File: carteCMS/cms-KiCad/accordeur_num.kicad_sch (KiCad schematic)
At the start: 16 parts, among them J2 Conn_01x16, J3 AVR-ISP-6, SW2 MCIPTG23K-V, SW3 MCIPTG23K-V, SW4 MCIPTG23K-V, U5 HP, U6 ATmega8U2-A, Y2 Crystal

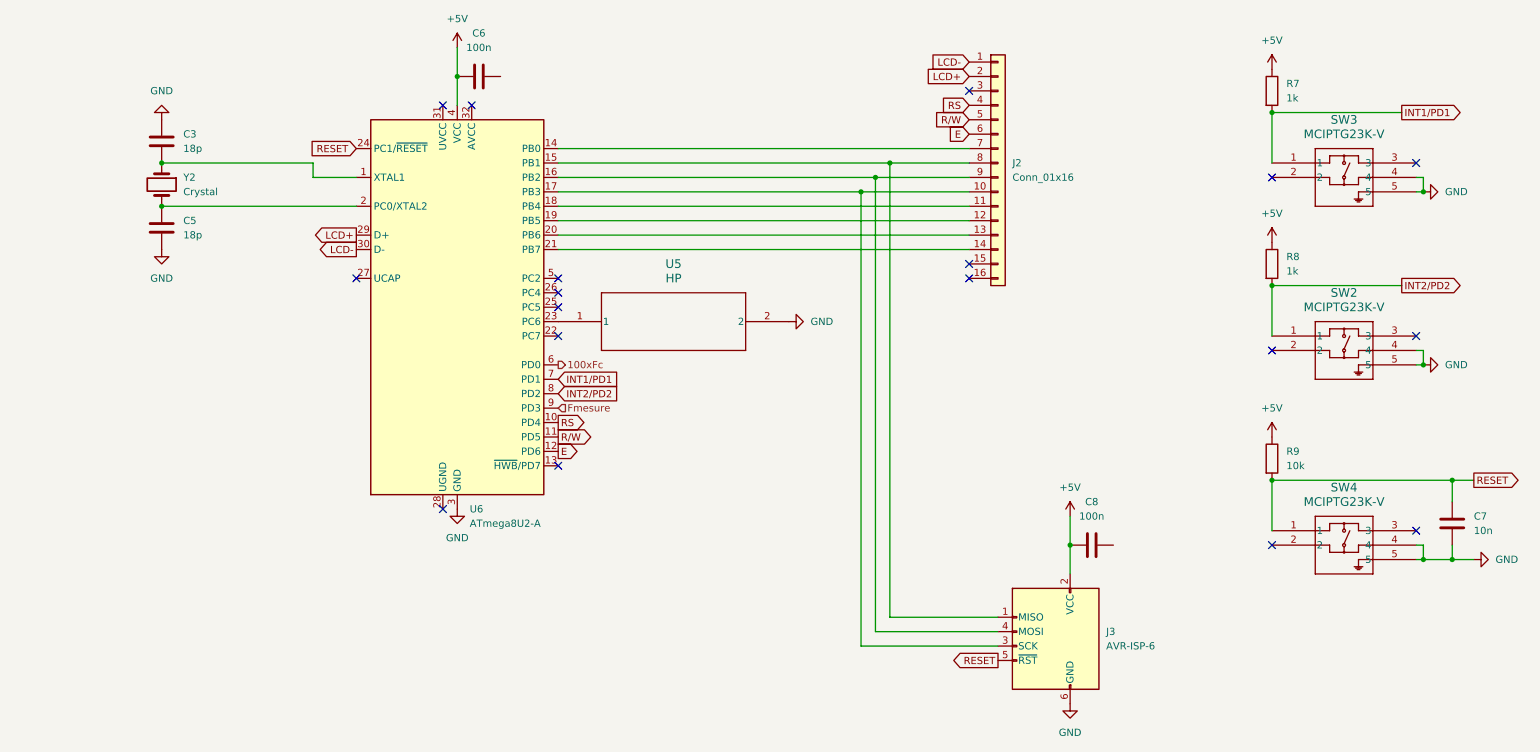
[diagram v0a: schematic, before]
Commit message: v2 - schéma et empruntes terminés (normalement)
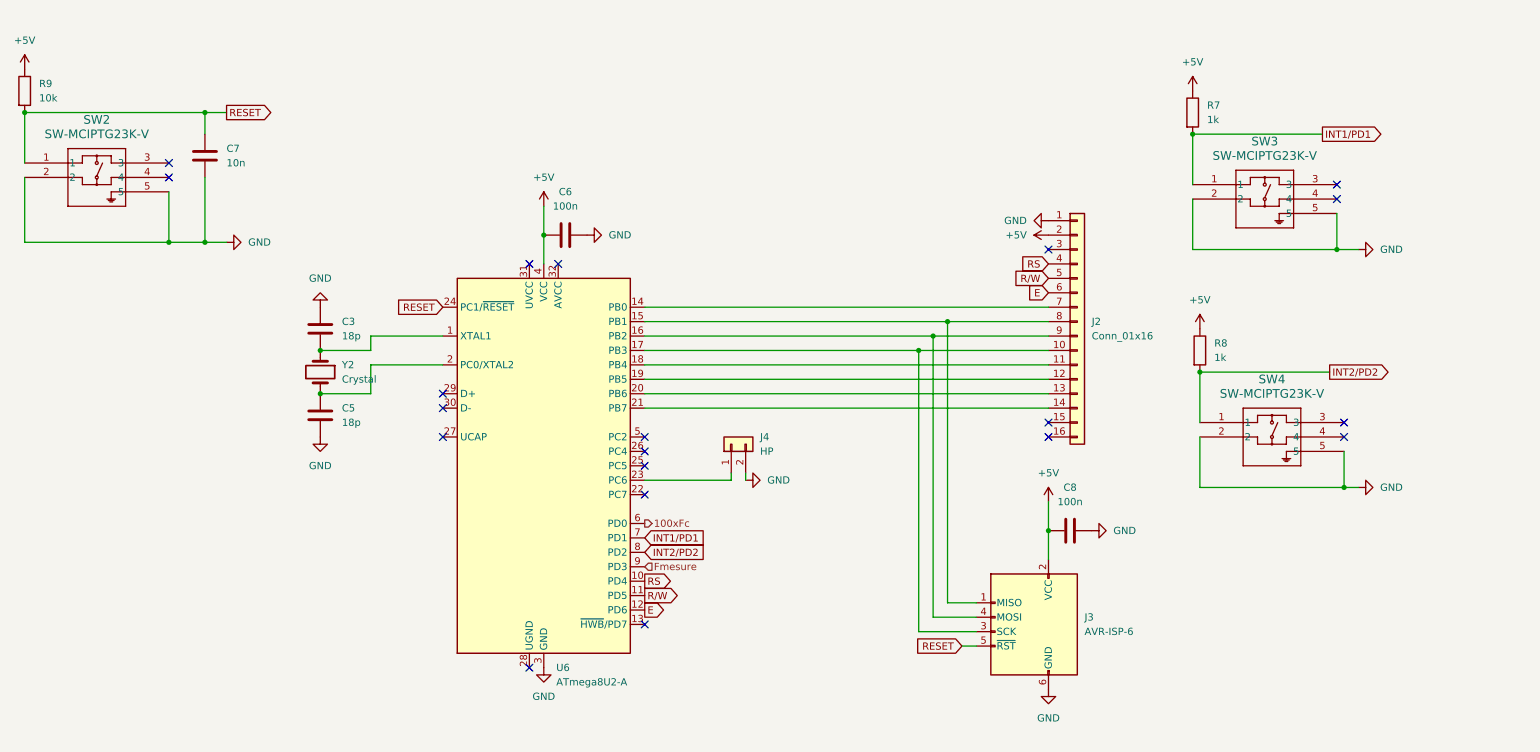
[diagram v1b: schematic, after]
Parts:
- removed SW2, SW3, SW4: MCIPTG23K-V, MCIPTG23K-V_MTC, symbol 2026-09-04_09-57-54:MCIPTG23K-V
- removed U5: HP, 2211S-02G_MTC, symbol 2026-09-04_10-13-27:HP
- added J4: HP, Connector_PinHeader_2.54mm:PinHeader_1x02_P2.54mm_Vertical, symbol Connector_Generic:Conn_01x02
- added SW2, SW3, SW4: SW-MCIPTG23K-V, accordeurEmp:SW-MCIPTG23K-V_MTC, symbol accordeurSym:SW-MCIPTG23K-V
- C3, C5, C6, C7, C8: footprint (none) -> Capacitor_SMD:C_0805_2012Metric
- J2: footprint (none) -> Connector_PinSocket_2.54mm:PinSocket_1x16_P2.54mm_Vertical
- J3: footprint (none) -> Connector_PinHeader_2.54mm:PinHeader_2x03_P2.54mm_Vertical
- Y2: footprint (none) -> accordeurEmp:quartz-HC49USMFB5F2016000MHZ
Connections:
- net +5V: now also J2.2 (Pin_2)
- net GND: now also C6.2, C8.2, J2.1 (Pin_1), J4.2 (Pin_2), SW2.2, SW2.5, SW3.2, SW3.5, SW4.2, SW4.5
- net INT1/PD1: now also SW3.1
- net INT2/PD2: now also SW4.1
- net RESET: now also SW2.1
- net at U6.23 (PC6): now also J4.1 (Pin_1)
- net LCD+: no longer names the net of U6.29 (D+)
- net LCD+: no longer J2.2 (Pin_2)
- net LCD-: no longer names the net of U6.30 (D-)
- net LCD-: no longer J2.1 (Pin_1)
- no-connect marks 18 -> 20
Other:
- moved on the sheet: C5, C6, C7, C8, J2, J3, R7, R8, R9, U6, Y2
